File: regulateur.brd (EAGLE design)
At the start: 41.9 x 29.2 mm, 15 parts, among them U1 LT1372CS8PBF

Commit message: Add files via upload
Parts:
- R1: value 12.76K -> 10K
- R2: value 37.24K -> 31.6K
- R3: value 5K -> 5.1K
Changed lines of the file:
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@@
 <element name="C5" library="resistor" package="CT7343" value="22uF" x="24.765" y="26.67" rot="R180"/>
 <element name="C1" library="resistor" package="CT7343" value="22uF" x="13.97" y="26.67" rot="R180"/>
-<element name="R1" library="resistor" package="R1206" value="12.76K" x="33.782" y="24.892"/>
-<element name="R2" library="resistor" package="R1206" value="37.24K" x="33.655" y="21.59" rot="R180"/>
-<element name="R3" library="resistor" package="R1206" value="5K" x="33.782" y="30.9245"/>
+<element name="R1" library="resistor" package="R1206" value="10K" x="33.782" y="24.892"/>
+<element name="R2" library="resistor" package="R1206" value="31.6K" x="33.655" y="21.59" rot="R180"/>
+<element name="R3" library="resistor" package="R1206" value="5.1K" x="33.782" y="30.9245"/>
 <element name="C2" library="resistor" package="C1206" value="10nF" x="39.37" y="33.655" rot="R180"/>
 <element name="C3" library="resistor" package="C1206" value="200pF" x="33.782" y="34.163" rot="R180"/>

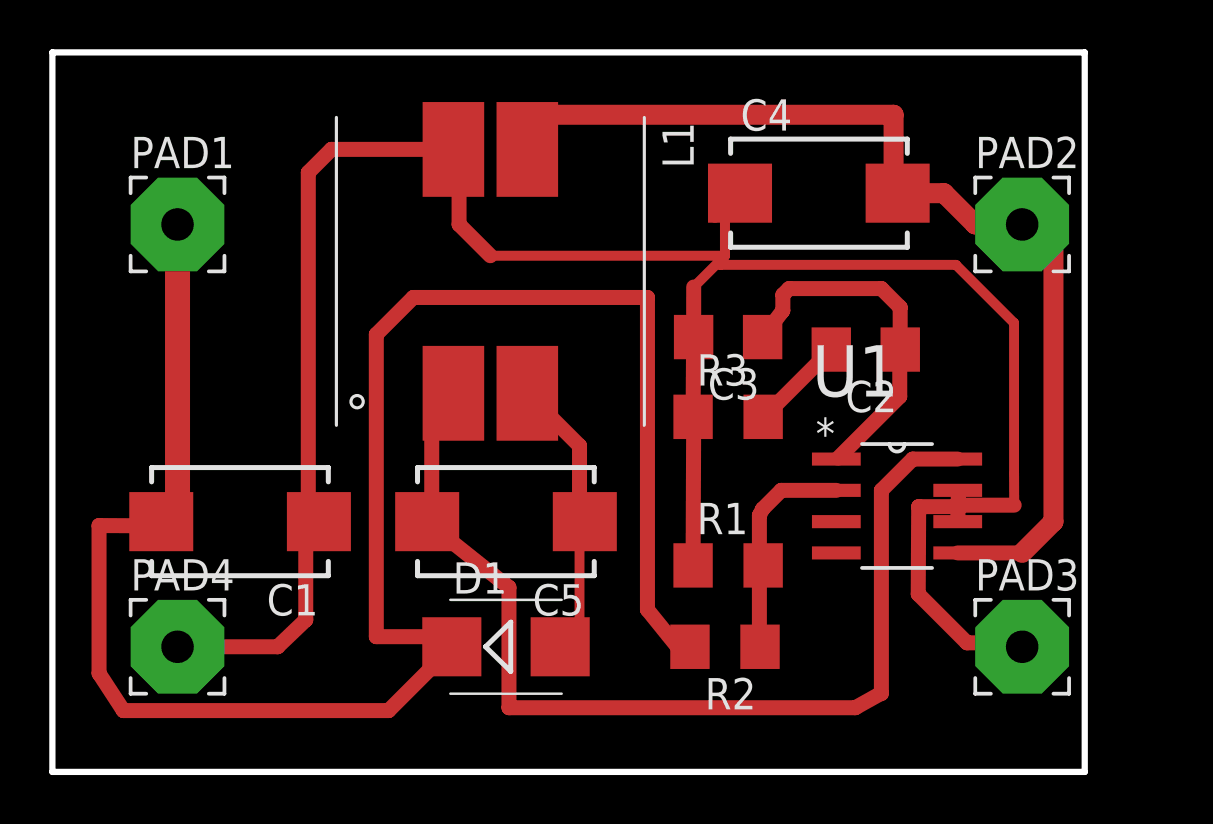
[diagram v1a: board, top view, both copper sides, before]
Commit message: Add files via upload
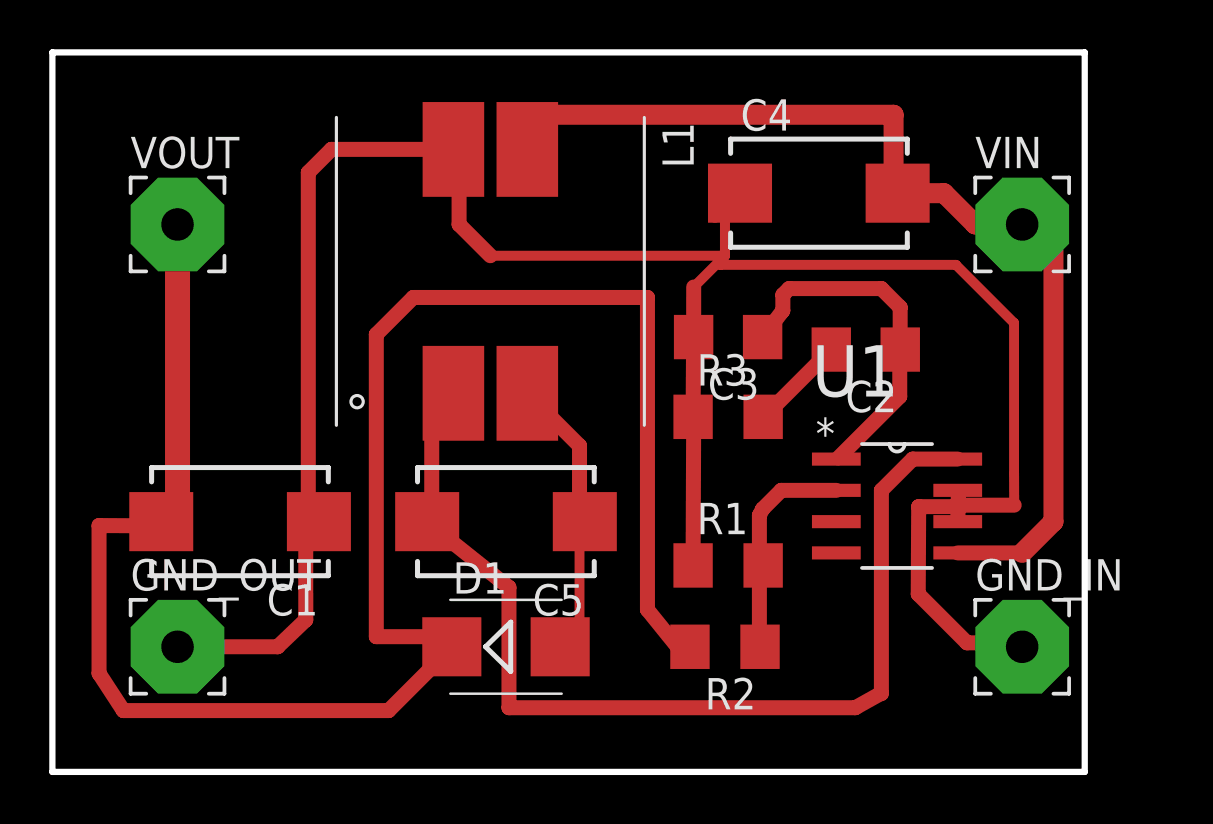
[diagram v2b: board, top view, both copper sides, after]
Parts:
- renumbered PAD1 to VOUT, PAD2 to VIN, PAD3 to GND_IN, PAD4 to GND_OUT
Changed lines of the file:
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@@
 <layer number="25" name="tNames" color="7" fill="1" visible="yes" active="yes"/>
 <layer number="26" name="bNames" color="7" fill="1" visible="no" active="yes"/>
-<layer number="27" name="tValues" color="7" fill="1" visible="yes" active="yes"/>
+<layer number="27" name="tValues" color="7" fill="1" visible="no" active="yes"/>
 <layer number="28" name="bValues" color="7" fill="1" visible="no" active="yes"/>
 <layer number="29" name="tStop" color="7" fill="3" visible="no" active="yes"/>
@@
 <layer number="39" name="tKeepout" color="4" fill="11" visible="no" active="yes"/>
 <layer number="40" name="bKeepout" color="1" fill="11" visible="no" active="yes"/>
-<layer number="41" name="tRestrict" color="4" fill="10" visible="yes" active="yes"/>
+<layer number="41" name="tRestrict" color="4" fill="10" visible="no" active="yes"/>
 <layer number="42" name="bRestrict" color="1" fill="10" visible="no" active="yes"/>
 <layer number="43" name="vRestrict" color="2" fill="10" visible="no" active="yes"/>
@@
 <element name="C2" library="resistor" package="C1206" value="10nF" x="39.37" y="33.655" rot="R180"/>
 <element name="C3" library="resistor" package="C1206" value="200pF" x="33.782" y="34.163" rot="R180"/>
-<element name="PAD1" library="wirepad" package="3,81/1,3" value="OUT" x="11.43" y="38.735"/>
-<element name="PAD2" library="wirepad" package="3,81/1,3" value="IN" x="45.72" y="38.735"/>
-<element name="PAD3" library="wirepad" package="3,81/1,3" value="IN_GND" x="45.72" y="21.59"/>
-<element name="PAD4" library="wirepad" package="3,81/1,3" value="OUT_GND" x="11.43" y="21.59"/>
+<element name="VOUT" library="wirepad" package="3,81/1,3" value="OUT" x="11.43" y="38.735"/>
+<element name="VIN" library="wirepad" package="3,81/1,3" value="IN" x="45.72" y="38.735"/>
+<element name="GND_IN" library="wirepad" package="3,81/1,3" value="IN_GND" x="45.72" y="21.59"/>
+<element name="GND_OUT" library="wirepad" package="3,81/1,3" value="OUT_GND" x="11.43" y="21.59"/>
 </elements>
 <signals>
@@
 <contactref element="C1" pad="+"/>
 <contactref element="R2" pad="2"/>
-<contactref element="PAD1" pad="1"/>
+<contactref element="VOUT" pad="1"/>
 <wire x1="22.5" y1="21.75" x2="22.565" y2="21.59" width="0.4032" layer="1"/>
 <wire x1="30.508" y1="23.095" x2="31.7236375" y2="21.5912375" width="0.6096" layer="1"/>
@@
 <contactref element="R1" pad="1"/>
 <contactref element="R3" pad="1"/>
-<contactref element="PAD3" pad="1"/>
-<contactref element="PAD4" pad="1"/>
+<contactref element="GND_IN" pad="1"/>
+<contactref element="GND_OUT" pad="1"/>
 <wire x1="43.128859375" y1="27.8466625" x2="43.1120625" y2="26.813340625" width="0.6096" layer="1"/>
 <wire x1="43.1120625" y1="26.813340625" x2="43.1038" y2="26.67" width="0.4032" layer="1"/>
@@
 <contactref element="U1" pad="5"/>
 <contactref element="L1" pad="3"/>
-<contactref element="PAD2" pad="1"/>
+<contactref element="VIN" pad="1"/>
 <wire x1="40.5" y1="43.187834375" x2="25.75" y2="43.187834375" width="0.8128" layer="1"/>
 <wire x1="40.5" y1="40.25" x2="40.5" y2="43.187834375" width="0.8128" layer="1"/>
